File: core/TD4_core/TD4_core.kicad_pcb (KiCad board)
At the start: 2 copper layers, 94 parts, among them J1 Conn_02x32_Row_Letter_First, J2 Conn_01x04, J3 Conn_01x04, J4 Conn_01x04, U1 74HC161, U10 74LS151, U11 74AHC1G04, U12 74AHC1G04, U13 74AHC1G86, U14 74AHC1G04, U15 74AHC1G86, U16 74HC86, U17 74HC04, U18 74HC21, U19 74HC86, U2 74HC161, U20 74HC04, U21 74HC86, U22 74HC04, U23 74HC86, U24 74HC04, U25 74HC21, U26 74HC86, U27 74HC04, U28 74HC21, U29 74HC153, U3 74HC161, U30 74HC153, U31 74HC74, U32 74HC175, U33 74AHC1G08, U34 74HC125, U35 74HC175, U36 74AHC1G08, U37 74HC155, U38 74HC125, U39 74HC125, U4 74HC161, U40 74HC125, U5 74HC86, U6 74HC08, U7 74HC32, U8 74HC86, U9 74HC08

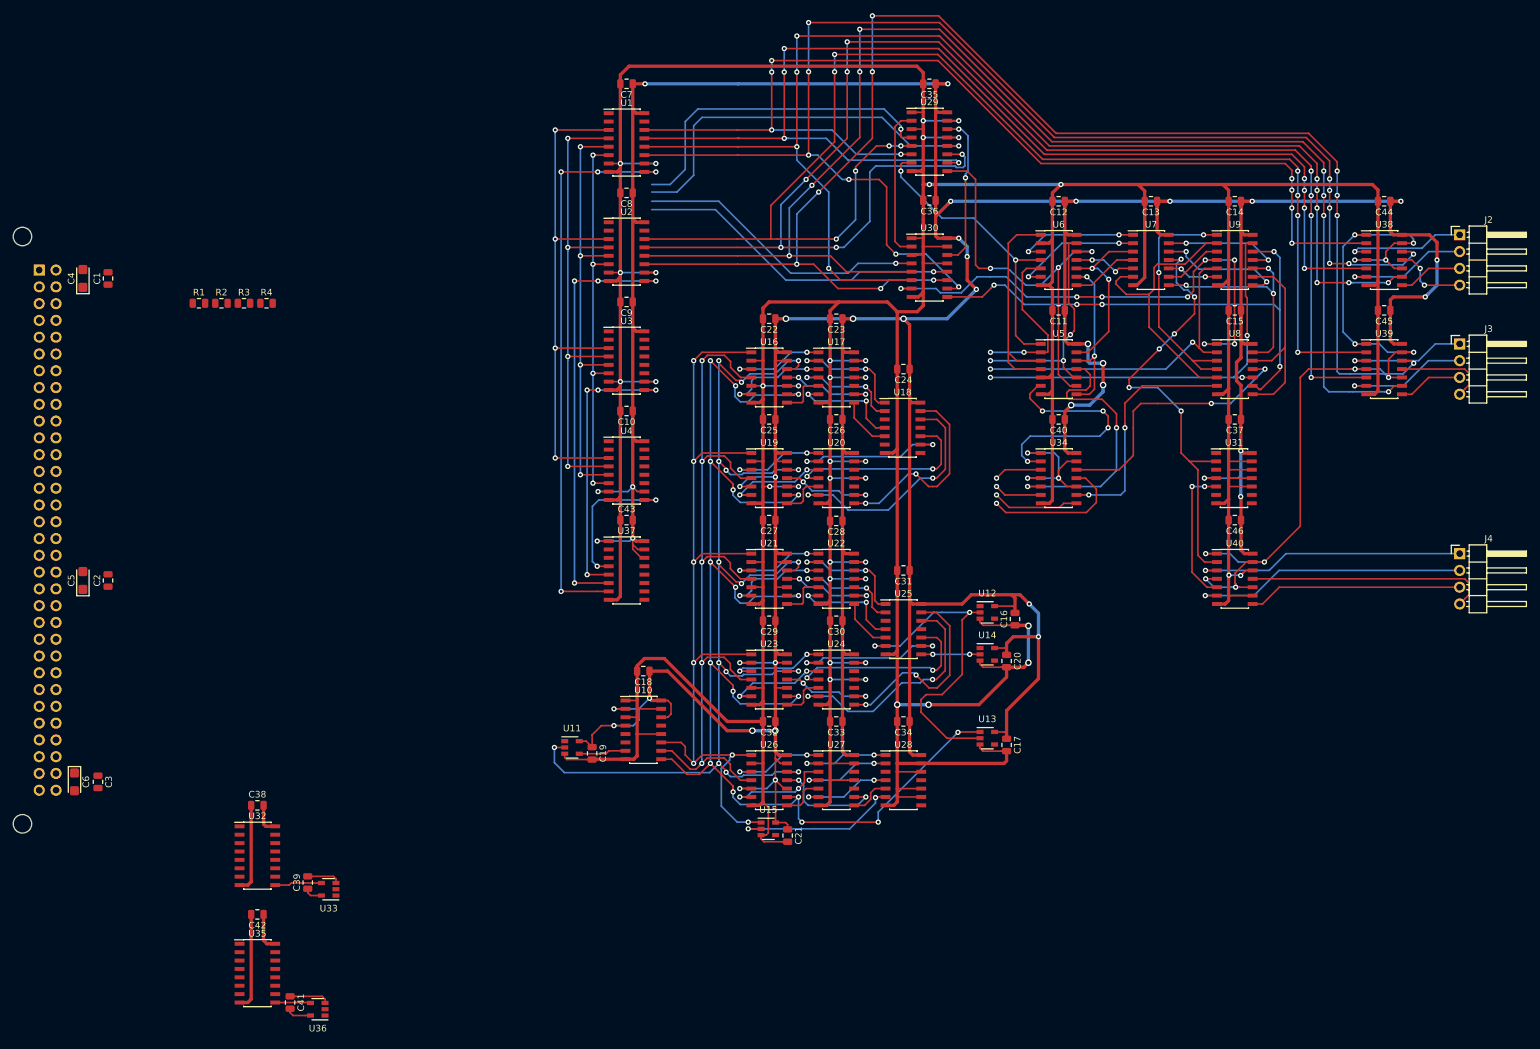
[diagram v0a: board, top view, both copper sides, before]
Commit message: Core routed
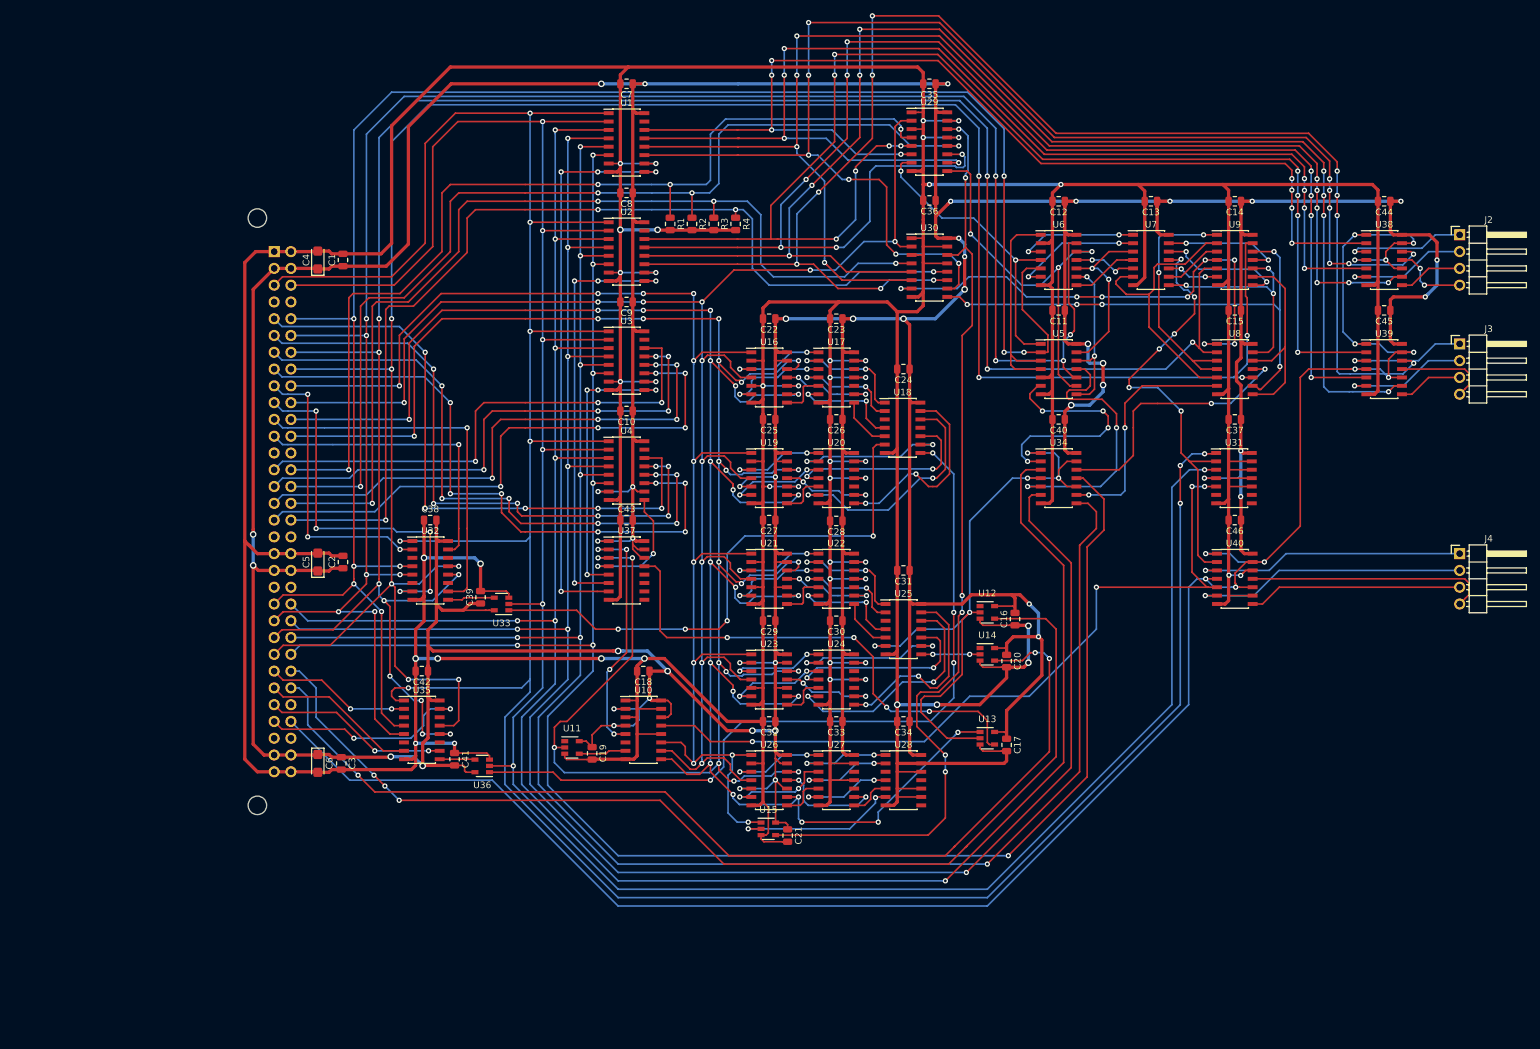
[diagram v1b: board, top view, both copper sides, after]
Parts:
- moved R1 72.3 mm to (123.4, 47.9), turned to 270 degrees
- moved R2 72.2 mm to (126.7, 47.9), turned to 270 degrees
- moved R3 72.1 mm to (130.0, 47.9), turned to 270 degrees
- moved R4 72.0 mm to (133.3, 47.9), turned to 270 degrees
- moved C39 50.5 mm to (94.7, 104.4)
- moved U33 50.5 mm to (97.9, 105.4)
- moved C38 50.5 mm to (87.1, 92.7)
- moved U32 50.5 mm to (87.1, 100.3)
- moved C41 44.5 mm to (90.8, 128.9)
- moved C42 44.5 mm to (85.9, 115.6)
- moved U36 44.5 mm to (95.0, 129.9)
- moved U35 44.5 mm to (85.9, 124.5)
- moved C3 36.9 mm to (73.7, 129.5)
- moved C6 36.9 mm to (70.1, 129.5)
- moved C1 35.7 mm to (73.9, 53.3)
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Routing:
- net ~RESET: track 0.00 -> 419.4 mm, vias 0 -> 9
- net CLK: track 0.00 -> 366.6 mm, vias 0 -> 7
- net GND: track 1054.8 -> 1340.2 mm, vias 38 -> 48
- net /RAM_A3: track 62.0 -> 344.0 mm, vias 3 -> 10
- net /RAM_A2: track 50.9 -> 330.6 mm, vias 2 -> 12
- net VCC: track 873.2 -> 1147.2 mm, vias 39 -> 46
- net /RAM_A1: track 34.7 -> 298.5 mm, vias 3 -> 10
- net /RAM_A0: track 25.4 -> 286.1 mm, vias 2 -> 8
- net /RAM_D0: track 89.3 -> 319.7 mm, vias 5 -> 7
- net /RAM_D1: track 81.6 -> 306.8 mm, vias 5 -> 7
- net /RAM_D2: track 79.9 -> 296.8 mm, vias 5 -> 7
- net /RAM_D3: track 81.2 -> 293.6 mm, vias 5 -> 7
- net /~DEBUG_ON~: track 139.4 -> 320.3 mm
- net /RAM_RW: track 0.00 -> 166.9 mm, vias 0 -> 3
- net /RAM_WE: track 0.00 -> 157.8 mm, vias 0 -> 3
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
